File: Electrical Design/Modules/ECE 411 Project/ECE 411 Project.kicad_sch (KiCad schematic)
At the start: 36 parts, among them J1 5mm 9V Barrel, J2 BOOST, J3 Pheonix Connector, SW1 SW_Push, SW2 SW_Push, SW3 SW_Push, SW4 SW_Push, SW5 SW_Push, SW6 SW_Push, SW7 SW_Push, SW8 SW_Push, U1 HT7333, U2 LT1054

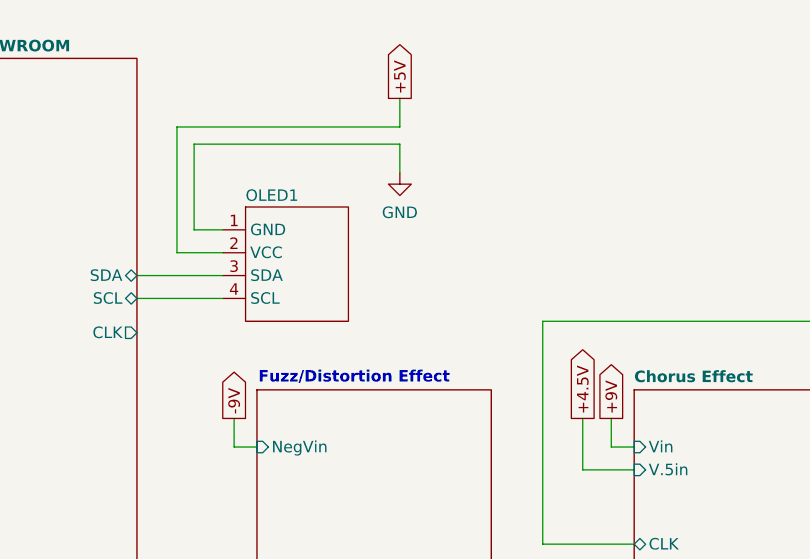
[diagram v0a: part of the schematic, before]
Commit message: update kicad
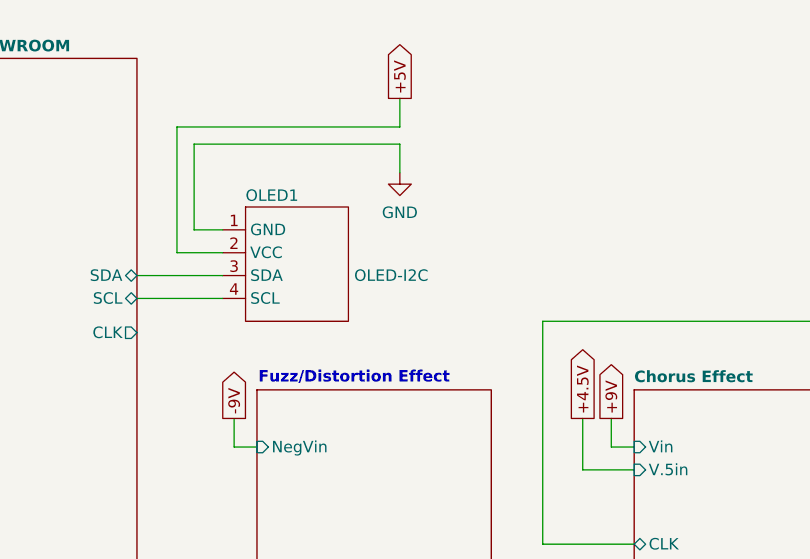
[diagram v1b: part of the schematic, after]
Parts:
- OLED1: value ~ -> OLED-I2C
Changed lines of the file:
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@@
 			)
 		)
-		(property "Value" "~"
+		(property "Value" "OLED-I2C"
 			(at 94.615 45.72 0)
 			(effects
